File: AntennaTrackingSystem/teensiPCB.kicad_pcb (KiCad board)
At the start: 2 copper layers, 45 x 84 mm, 13 parts, among them J1 screw terminal, J2 Conn_01x02, J5 UART1, J6 UART2, J7 I2C ext, SW1 SW_Push, U1 Teensy4.1, U2 SAM-M10Q-00B

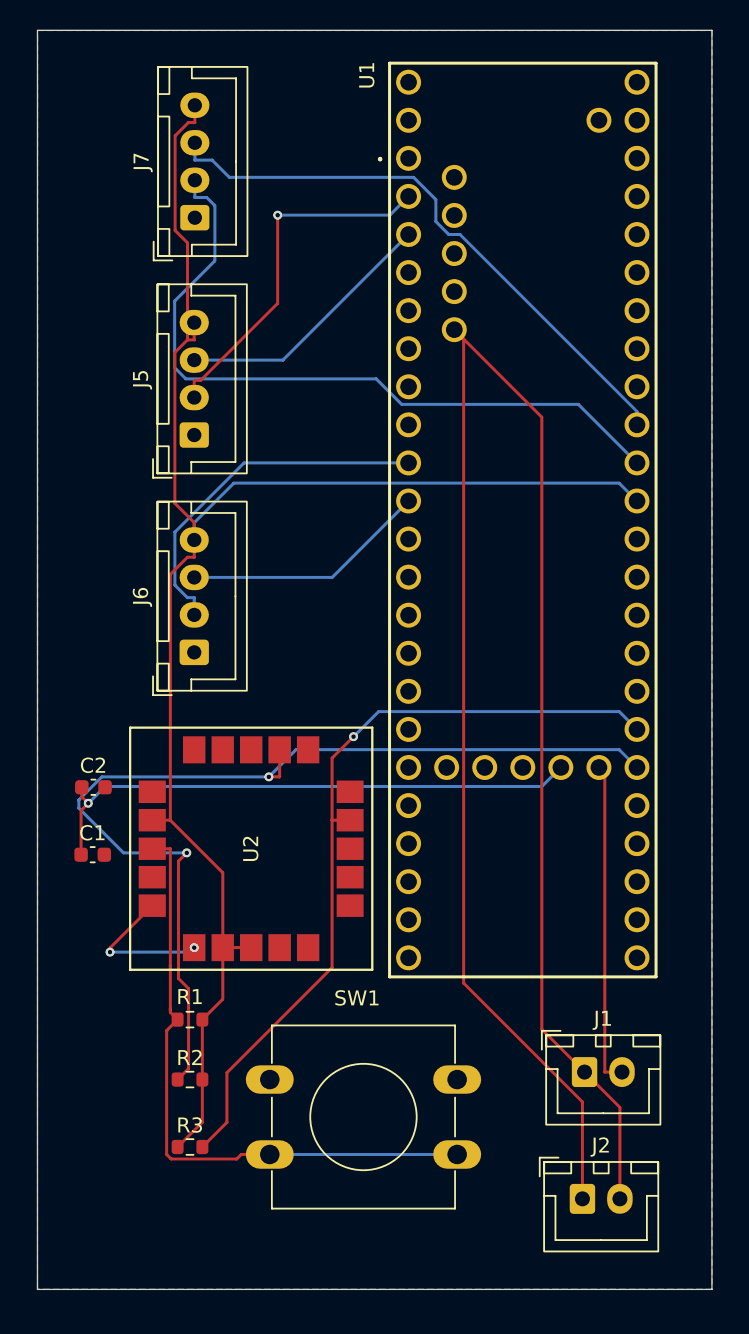
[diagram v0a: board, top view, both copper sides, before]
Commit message: update pcb slightly
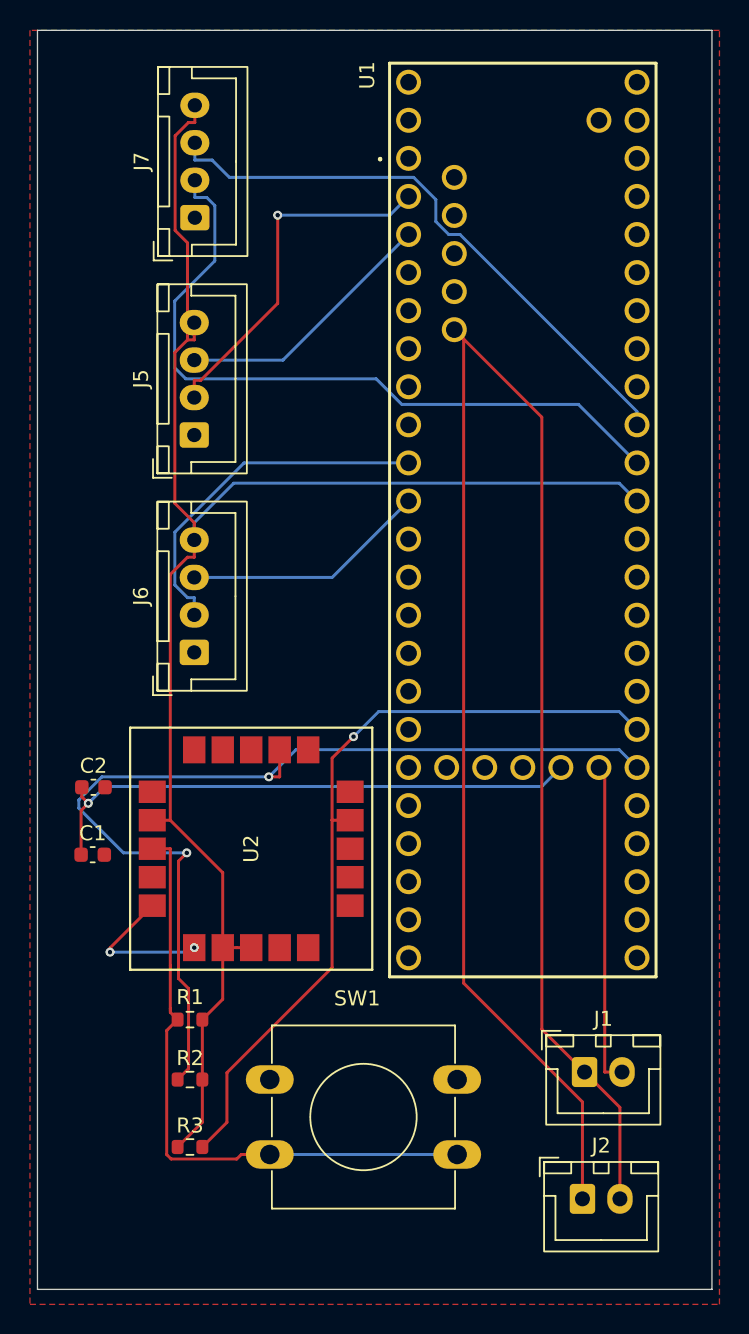
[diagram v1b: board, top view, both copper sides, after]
